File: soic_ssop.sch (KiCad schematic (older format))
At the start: 2 parts, among them P8 CONN_8, P9 CONN_8

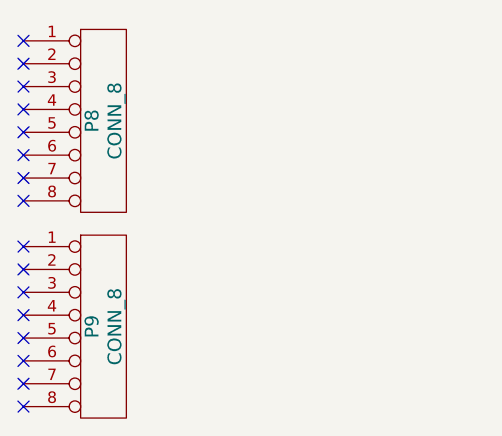
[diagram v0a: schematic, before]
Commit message: ftdi done + breakout done
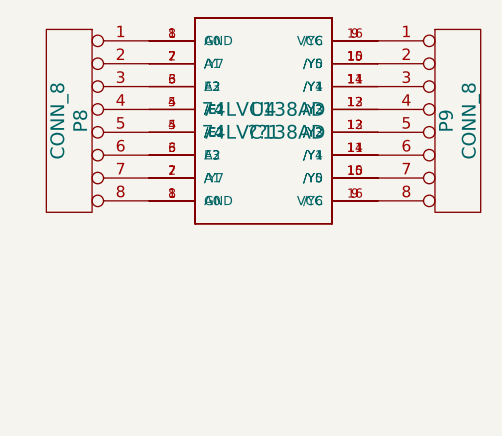
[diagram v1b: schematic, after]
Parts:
- added ??1, U4: 74LVC138AD, ~, symbol 74LVC138AD
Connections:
- net at P8.1 (P1): now also ??1.8 (GND), U4.1 (A0)
- net at P8.2 (P2): now also ??1.7 (/Y7), U4.2 (A1)
- net at P8.3 (P3): now also ??1.6 (E3), U4.3 (A2)
- net at P8.4 (P4): now also ??1.5 (/E2), U4.4 (/E1)
- net at P8.5 (P5): now also ??1.4 (/E1), U4.5 (/E2)
- net at P8.6 (P6): now also ??1.3 (A2), U4.6 (E3)
- net at P8.7 (P7): now also ??1.2 (A1), U4.7 (/Y7)
- net at P8.8 (P8): now also ??1.1 (A0), U4.8 (GND)
- net at P9.1 (P1): now also ??1.9 (/Y6), U4.16 (VCC)
- net at P9.2 (P2): now also ??1.10 (/Y5), U4.15 (/Y0)
- net at P9.3 (P3): now also ??1.11 (/Y4), U4.14 (/Y1)
- net at P9.4 (P4): now also ??1.12 (/Y3), U4.13 (/Y2)
- net at P9.5 (P5): now also ??1.13 (/Y2), U4.12 (/Y3)
- net at P9.6 (P6): now also ??1.14 (/Y1), U4.11 (/Y4)
- net at P9.7 (P7): now also ??1.15 (/Y0), U4.10 (/Y5)
- net at P9.8 (P8): now also ??1.16 (VCC), U4.9 (/Y6)
- no-connect marks 16 -> 0
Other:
- moved on the sheet: P8, P9
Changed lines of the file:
@@
-EESchema Schematic File Version 2
+EESchema Schematic File Version 2  date 03-08-2013 21:17:06
 LIBS:power
 LIBS:device
@@
 L CONN_8 P8
 U 1 1 51FCB26D
-P 3400 2600
-F 0 "P8" V 3350 2600 60  0000 C CNN
-F 1 "CONN_8" V 3450 2600 60  0000 C CNN
-F 2 "" H 3400 2600 60  0000 C CNN
-F 3 "" H 3400 2600 60  0000 C CNN
-	1    3400 2600
-	1    0    0    -1
+P 3250 2600
+F 0 "P8" V 3200 2600 60  0000 C CNN
+F 1 "CONN_8" V 3300 2600 60  0000 C CNN
+F 2 "" H 3250 2600 60  0000 C CNN
+F 3 "" H 3250 2600 60  0000 C CNN
+	1    3250 2600
+	-1   0    0    -1
 $EndComp
 $Comp
 L CONN_8 P9
 U 1 1 51FCB27C
-P 3400 3500
-F 0 "P9" V 3350 3500 60  0000 C CNN
-F 1 "CONN_8" V 3450 3500 60  0000 C CNN
-F 2 "" H 3400 3500 60  0000 C CNN
-F 3 "" H 3400 3500 60  0000 C CNN
-	1    3400 3500
+P 4950 2600
+F 0 "P9" V 4900 2600 60  0000 C CNN
+F 1 "CONN_8" V 5000 2600 60  0000 C CNN
+F 2 "" H 4950 2600 60  0000 C CNN
+F 3 "" H 4950 2600 60  0000 C CNN
+	1    4950 2600
 	1    0    0    -1
 $EndComp
-NoConn ~ 3050 2250
-NoConn ~ 3050 2350
-NoConn ~ 3050 2450
-NoConn ~ 3050 2550
-NoConn ~ 3050 2650
-NoConn ~ 3050 2750
-NoConn ~ 3050 2850
-NoConn ~ 3050 2950
-NoConn ~ 3050 3150
-NoConn ~ 3050 3250
-NoConn ~ 3050 3350
-NoConn ~ 3050 3450
-NoConn ~ 3050 3550
-NoConn ~ 3050 3650
-NoConn ~ 3050 3750
-NoConn ~ 3050 3850
+$Comp
+L 74LVC138AD ??1
+U 1 1 51FD6D10
+P 4100 2650
+F 0 "??1" H 4100 2650 60  0000 C CNN
+F 1 "74LVC138AD" H 4100 2650 60  0000 C CNN
+F 2 "~" H 4100 2650 60  0000 C CNN
+F 3 "~" H 4100 2650 60  0000 C CNN
+	1    4100 2650
+	1    0    0    1
+$EndComp
+$Comp
+L 74LVC138AD U4
+U 1 1 51FD6D1D
+P 4100 2550
+F 0 "U4" H 4100 2550 60  0000 C CNN
+F 1 "74LVC138AD" H 4100 2550 60  0000 C CNN
+F 2 "~" H 4100 2550 60  0000 C CNN
+F 3 "~" H 4100 2550 60  0000 C CNN
+	1    4100 2550
+	1    0    0    -1
+$EndComp
 $EndSCHEMATC
